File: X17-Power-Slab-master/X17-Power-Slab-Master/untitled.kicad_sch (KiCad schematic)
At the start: 5 parts

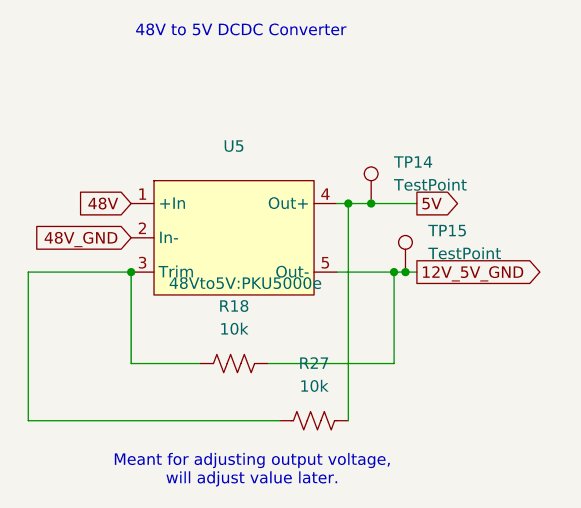
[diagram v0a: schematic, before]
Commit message: final for 12/30 meeting
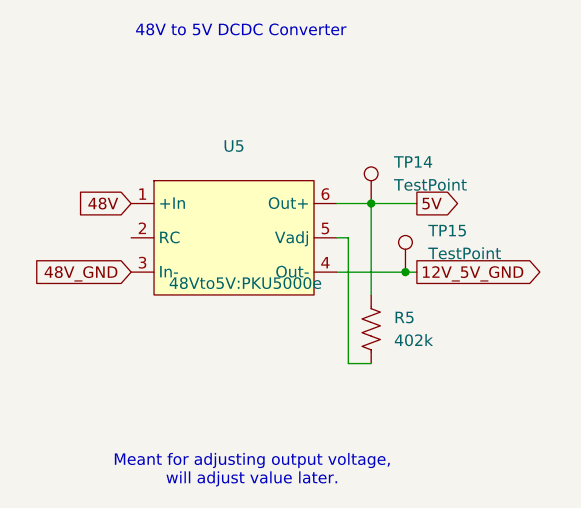
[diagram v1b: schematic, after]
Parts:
- removed R18, R27: 10k, Resistor_SMD:R_0603_1608Metric_Pad0.98x0.95mm_HandSolder, symbol Device:R_US
- added R5: 402k, Resistor_SMD:R_0603_1608Metric_Pad0.98x0.95mm_HandSolder, symbol Device:R_US
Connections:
- net 12V_5V_GND: now also U5.4 (Out-); no longer U5.5 (Out-)
- net 48V_GND: now also U5.3 (In-); no longer U5.2 (In-)
- net 5V: now also U5.6 (Out+), R5.1; no longer U5.4 (Out+)
- new net: R5.2, U5.5 (Vadj)
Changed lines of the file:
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@@
-	)
-	(junction
-		(at 109.22 87.63)
-		(diameter 0)
-		(color 0 0 0 0)
-	)
-	(junction
-		(at 133.35 80.01)
-		(diameter 0)
-		(color 0 0 0 0)
 	)
 	(junction
@@
 		(color 0 0 0 0)
 	)
-	(junction
-		(at 138.43 87.63)
-		(diameter 0)
-		(color 0 0 0 0)
-	)
-	(wire
-		(pts
-			(xy 124.46 97.79) (xy 138.43 97.79)
-		)
-		(stroke
-			(width 0)
-			(type default)
-		)
-	)
-	(wire
-		(pts
-			(xy 109.22 97.79) (xy 116.84 97.79)
+	(wire
+		(pts
+			(xy 133.35 97.79) (xy 135.89 97.79)
 		)
 		(stroke
@@
 	(wire
 		(pts
-			(xy 132.08 87.63) (xy 138.43 87.63)
-		)
-		(stroke
-			(width 0)
-			(type default)
-		)
-	)
-	(wire
-		(pts
-			(xy 97.79 87.63) (xy 97.79 104.14)
-		)
-		(stroke
-			(width 0)
-			(type default)
-		)
-	)
-	(wire
-		(pts
-			(xy 109.22 87.63) (xy 109.22 97.79)
-		)
-		(stroke
-			(width 0)
-			(type default)
-		)
-	)
-	(wire
-		(pts
-			(xy 133.35 80.01) (xy 133.35 104.14)
-		)
-		(stroke
-			(width 0)
-			(type default)
-		)
-	)
-	(wire
-		(pts
-			(xy 138.43 87.63) (xy 138.43 97.79)
-		)
-		(stroke
-			(width 0)
-			(type default)
-		)
-	)
-	(wire
-		(pts
-			(xy 97.79 87.63) (xy 109.22 87.63)
-		)
-		(stroke
-			(width 0)
-			(type default)
-		)
-	)
-	(wire
-		(pts
-			(xy 97.79 104.14) (xy 125.73 104.14)
-		)
-		(stroke
-			(width 0)
-			(type default)
-		)
-	)
-	(wire
-		(pts
-			(xy 138.43 87.63) (xy 139.7 87.63)
-		)
-		(stroke
-			(width 0)
-			(type default)
-		)
-	)
-	(wire
-		(pts
-			(xy 132.08 80.01) (xy 133.35 80.01)
+			(xy 132.08 83.82) (xy 133.35 83.82)
+		)
+		(stroke
+			(width 0)
+			(type default)
+		)
+	)
+	(wire
+		(pts
+			(xy 132.08 87.63) (xy 139.7 87.63)
+		)
+		(stroke
+			(width 0)
+			(type default)
+		)
+	)
+	(wire
+		(pts
+			(xy 133.35 83.82) (xy 133.35 97.79)
+		)
+		(stroke
+			(width 0)
+			(type default)
+		)
+	)
+	(wire
+		(pts
+			(xy 135.89 80.01) (xy 135.89 90.17)
+		)
+		(stroke
+			(width 0)
+			(type default)
+		)
+	)
+	(wire
+		(pts
+			(xy 132.08 80.01) (xy 135.89 80.01)
 		)
 		(stroke
@@
 		)
 	)
-	(wire
-		(pts
-			(xy 133.35 80.01) (xy 135.89 80.01)
-		)
-		(stroke
-			(width 0)
-			(type default)
-		)
-	)
 	(text "Meant for adjusting output voltage, \nwill adjust value later."
 		(exclude_from_sim no)
@@
 			(font
 				(size 1.27 1.27)
+			)
+		)
+	)
+	(global_label "48V_GND"
+		(shape input)
+		(at 109.22 87.63 180)
+		(fields_autoplaced yes)
+		(effects
+			(font
+				(size 1.27 1.27)
+			)
+			(justify right)
+		)
+		(property "Intersheetrefs" "${INTERSHEET_REFS}"
+			(at 97.8891 87.63 0)
+			(effects
+				(font
+					(size 1.27 1.27)
+				)
+				(justify right)
+				(hide yes)
 			)
 		)
@@
 				)
 				(justify left)
-				(hide yes)
-			)
-		)
-	)
-	(global_label "48V_GND"
-		(shape input)
-		(at 109.22 83.82 180)
-		(fields_autoplaced yes)
-		(effects
-			(font
-				(size 1.27 1.27)
-			)
-			(justify right)
-		)
-		(property "Intersheetrefs" "${INTERSHEET_REFS}"
-			(at 97.8891 83.82 0)
-			(effects
-				(font
-					(size 1.27 1.27)
-				)
-				(justify right)
 				(hide yes)
 			)
@@
 	(symbol
 		(lib_id "Device:R_US")
-		(at 129.54 104.14 270)
+		(at 135.89 93.98 0)
 		(unit 1)
 		(exclude_from_sim no)
@@
 		(dnp no)
 		(fields_autoplaced yes)
-		(property "Reference" "R27"
-			(at 129.54 97.79 90)
-			(effects
-				(font
-					(size 1.27 1.27)
-				)
-			)
-		)
-		(property "Value" "10k"
-			(at 129.54 100.33 90)
-			(effects
-				(font
-					(size 1.27 1.27)
-				)
+		(property "Reference" "R5"
+			(at 138.43 92.7099 0)
+			(effects
+				(font
+					(size 1.27 1.27)
+				)
+				(justify left)
+			)
+		)
+		(property "Value" "402k"
+			(at 138.43 95.2499 0)
+			(effects
+				(font
+					(size 1.27 1.27)
+				)
+				(justify left)
 			)
 		)
 		(property "Footprint" "Resistor_SMD:R_0603_1608Metric_Pad0.98x0.95mm_HandSolder"
-			(at 129.286 105.156 90)
+			(at 136.906 94.234 90)
 			(effects
 				(font
@@
 		)
 		(property "Datasheet" "~"
-			(at 129.54 104.14 0)
+			(at 135.89 93.98 0)
 			(effects
 				(font
@@
 		)
 		(property "Description" "Resistor, US symbol"
-			(at 129.54 104.14 0)
-			(effects
-				(font
-					(size 1.27 1.27)
-				)
-				(hide yes)
-			)
-		)
-		(pin "1"
-		)
-		(pin "2"
-		)
-		(instances
-			(project "X17-Power-Slab-Master"
-				(path "/57e59c68-7be1-495e-b535-e78e0f561e15/bdfdae5a-9acb-4759-8fe8-e68c48f1ce0d"
-					(reference "R27")
-					(unit 1)
-				)
-			)
-		)
-	)
-	(symbol
-		(lib_id "Device:R_US")
-		(at 120.65 97.79 270)
-		(unit 1)
-		(exclude_from_sim no)
-		(in_bom yes)
-		(on_board yes)
-		(dnp no)
-		(fields_autoplaced yes)
-		(property "Reference" "R18"
-			(at 120.65 91.44 90)
-			(effects
-				(font
-					(size 1.27 1.27)
-				)
-			)
-		)
-		(property "Value" "10k"
-			(at 120.65 93.98 90)
-			(effects
-				(font
-					(size 1.27 1.27)
-				)
-			)
-		)
-		(property "Footprint" "Resistor_SMD:R_0603_1608Metric_Pad0.98x0.95mm_HandSolder"
-			(at 120.396 98.806 90)
-			(effects
-				(font
-					(size 1.27 1.27)
-				)
-				(hide yes)
-			)
-		)
-		(property "Datasheet" "~"
-			(at 120.65 97.79 0)
-			(effects
-				(font
-					(size 1.27 1.27)
-				)
-				(hide yes)
-			)
-		)
-		(property "Description" "Resistor, US symbol"
-			(at 120.65 97.79 0)
+			(at 135.89 93.98 0)
 			(effects
 				(font
@@
 			(project ""
 				(path "/57e59c68-7be1-495e-b535-e78e0f561e15/bdfdae5a-9acb-4759-8fe8-e68c48f1ce0d"
-					(reference "R18")
+					(reference "R5")
 					(unit 1)
 				)
@@
 		(pin "2"
 		)
+		(pin "6"
+		)
 		(instances
